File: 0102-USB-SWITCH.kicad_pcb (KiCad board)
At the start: 2 copper layers, 39.6 x 24.6 mm, 20 parts, among them J1 UPSTREAM, J2 DOWNSTREAM, SW1 EN

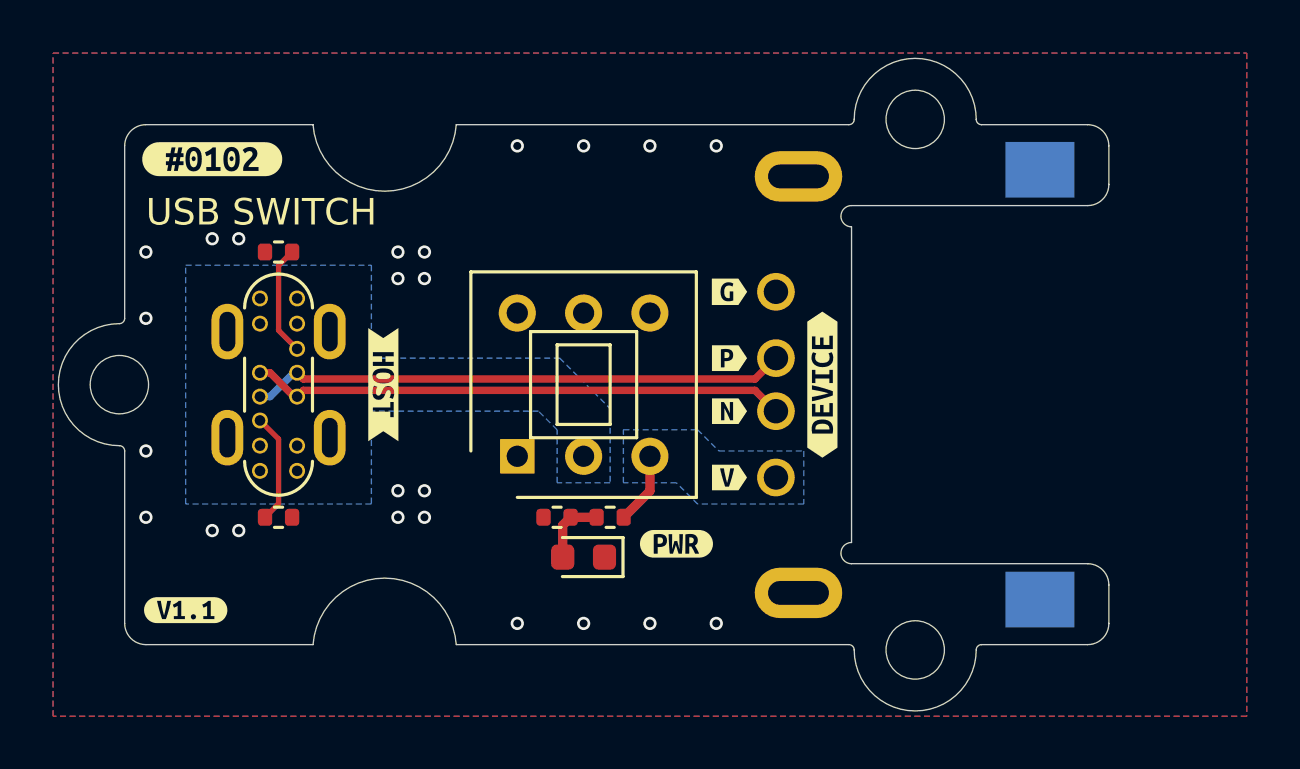
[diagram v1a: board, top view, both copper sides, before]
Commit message: Rework with new design
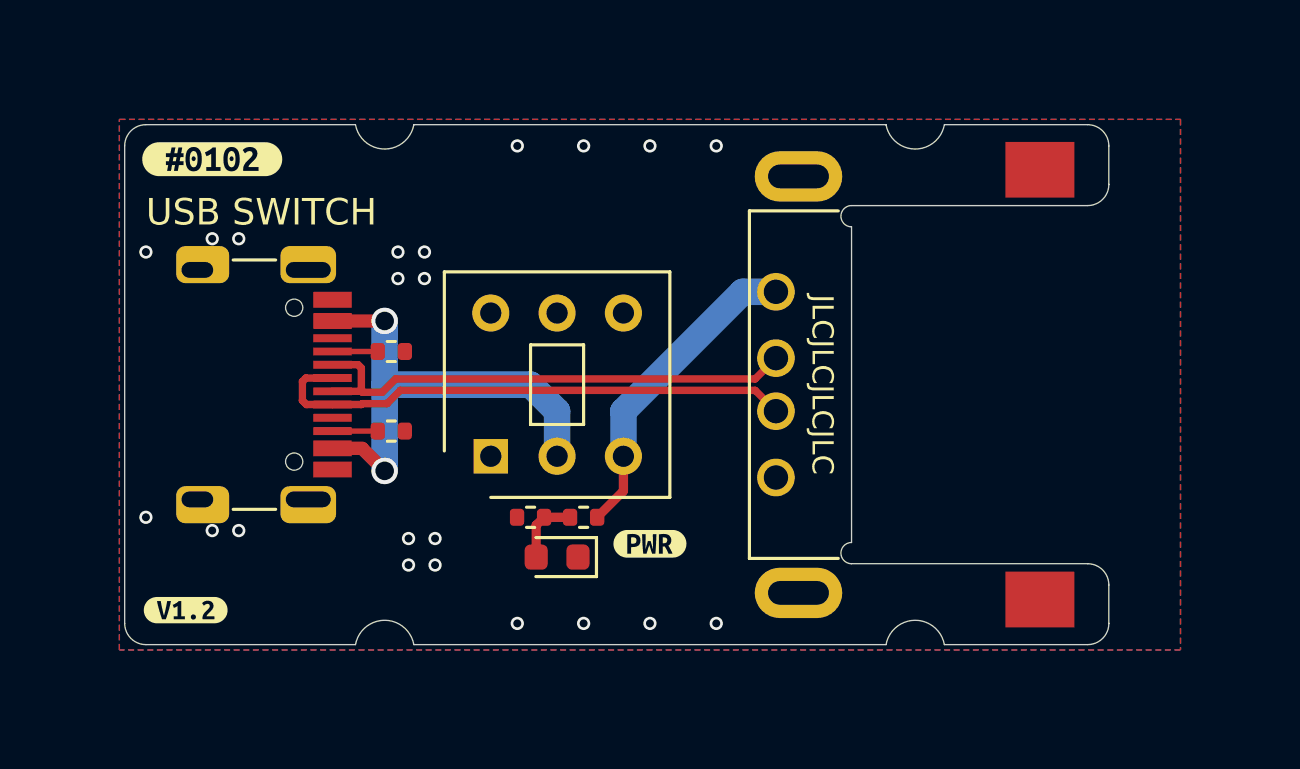
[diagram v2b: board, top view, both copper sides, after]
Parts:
- removed H1, H2, H3: MountingHole, MountingHole:MountingHole_2.2mm_M2
- removed kibuzzard-631FFD46: G***, kibuzzard-631FFD46
- removed kibuzzard-631FFF00: G***, kibuzzard-631FFF00
- removed kibuzzard-631FFF07: G***, kibuzzard-631FFF07
- removed kibuzzard-63200097: G***, kibuzzard-63200097
- removed kibuzzard-6320009C: G***, kibuzzard-6320009C
- removed kibuzzard-632000A0: G***, kibuzzard-632000A0
- removed kibuzzard-632000A4: G***, kibuzzard-632000A4
- added kibuzzard-632D82D3: G***, kibuzzard-632D82D3, B.Cu at (123.0, 106.5)
- added kibuzzard-632D82DD: G***, kibuzzard-632D82DD, B.Cu at (123.0, 109.0)
- added kibuzzard-632D82E6: G***, kibuzzard-632D82E6, B.Cu at (123.0, 111.0)
- added kibuzzard-632D82EF: G***, kibuzzard-632D82EF, B.Cu at (123.0, 113.5)
- added kibuzzard-632D83AE: G***, kibuzzard-632D83AE, F.Cu at (102.5, 118.5)
- J1: footprint JLC-SMT:KINGHELM_KH-TYPE-C-L10-14P -> JLC-SMT:HRO_TYPE-C-31-M-12
- J2: moved to F.Cu
- moved R4 7.98 mm to (110.2, 111.8), turned to 180 degrees
- moved R3 7.56 mm to (110.2, 108.8)
- moved J1 2.01 mm to (104.0, 110.0), turned to -90 degrees
- moved D1 1.00 mm to (116.5, 116.5)
- moved R1 1.00 mm to (117.5, 115.0)
- moved R2 1.00 mm to (115.5, 115.0)
- moved SW1 1.00 mm to (116.5, 110.0)
- moved kibuzzard-631FFEA9 1.00 mm to (120.0, 116.0)
- turned J2 to 90 degrees
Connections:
- J1 pad S1: unconnected-(J1-PadS1) -> GND
- J2 pad 5: unconnected-(J2-Pad5) -> GND
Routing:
- net /VIN: track 0.00 -> 18.5 mm, vias 0 -> 2
- net /VOUT: track 2.71 -> 12.0 mm
- net Net-(J1-PadB5): track 4.15 -> 1.70 mm
- net Net-(J1-PadA5): track 4.15 -> 1.70 mm
- net /D-: track 20.2 -> 19.3 mm
- net GND: vias 24 -> 22
- removed copper zone on B.Cu, net /VIN
- removed copper zone on B.Cu, net /VOUT
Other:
- board size 39.6 x 24.6 mm -> 37.1 x 19.6 mm
